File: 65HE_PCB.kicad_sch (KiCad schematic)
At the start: 30 parts, among them J001 JST_SH, SW1 BOOT, SW2 NRST, U201 TLV75733PDBV, U202 TLV75733PDBV, U301 STM32F072CBTx

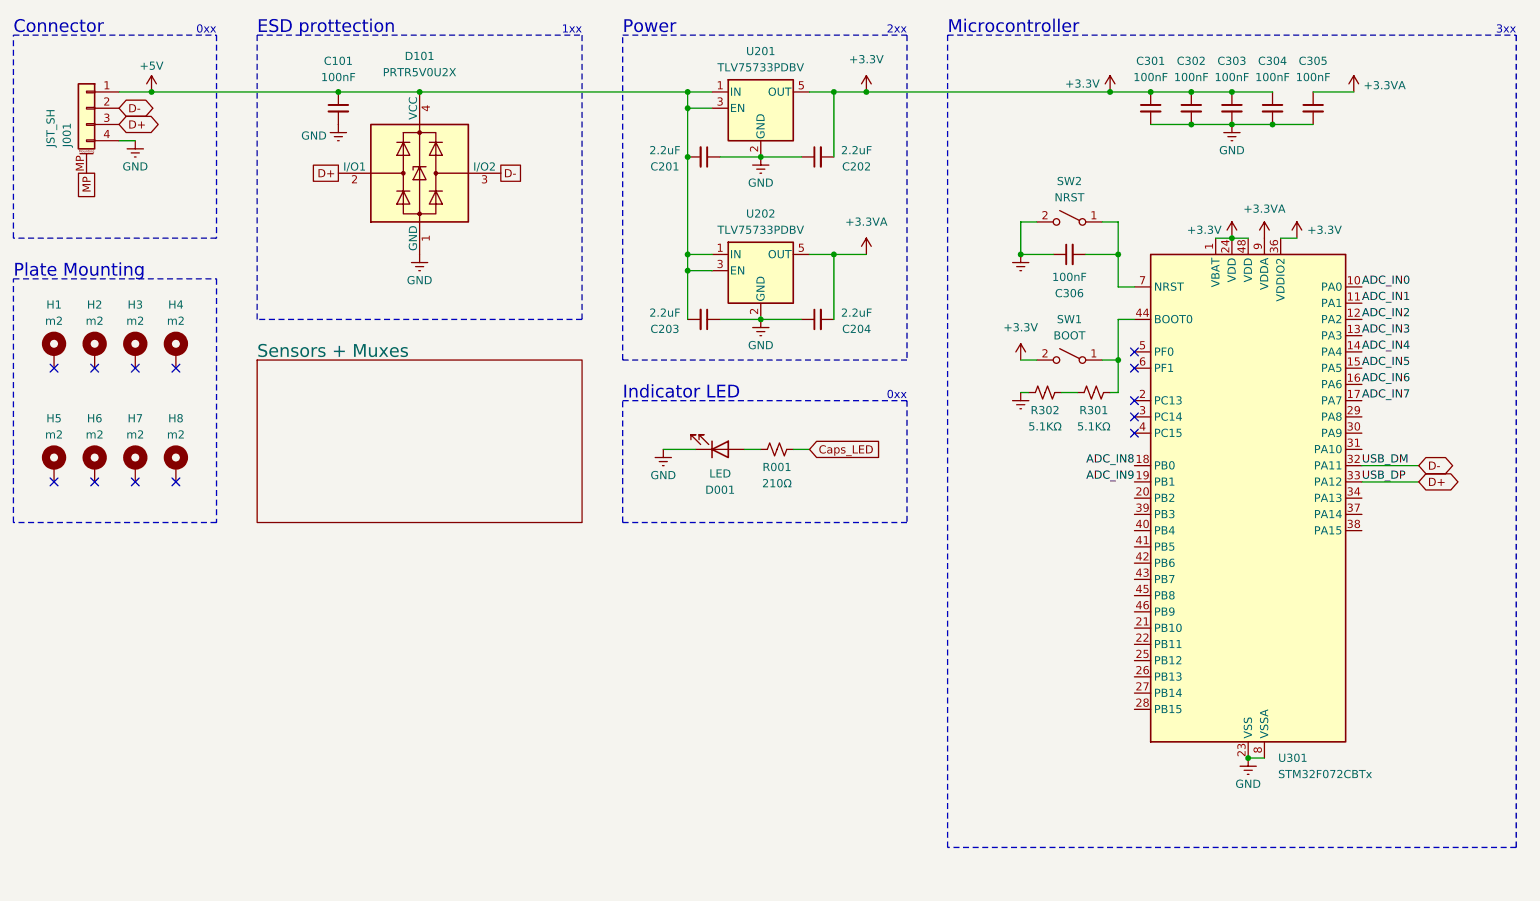
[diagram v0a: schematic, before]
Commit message: initial commit
i made the board yay!
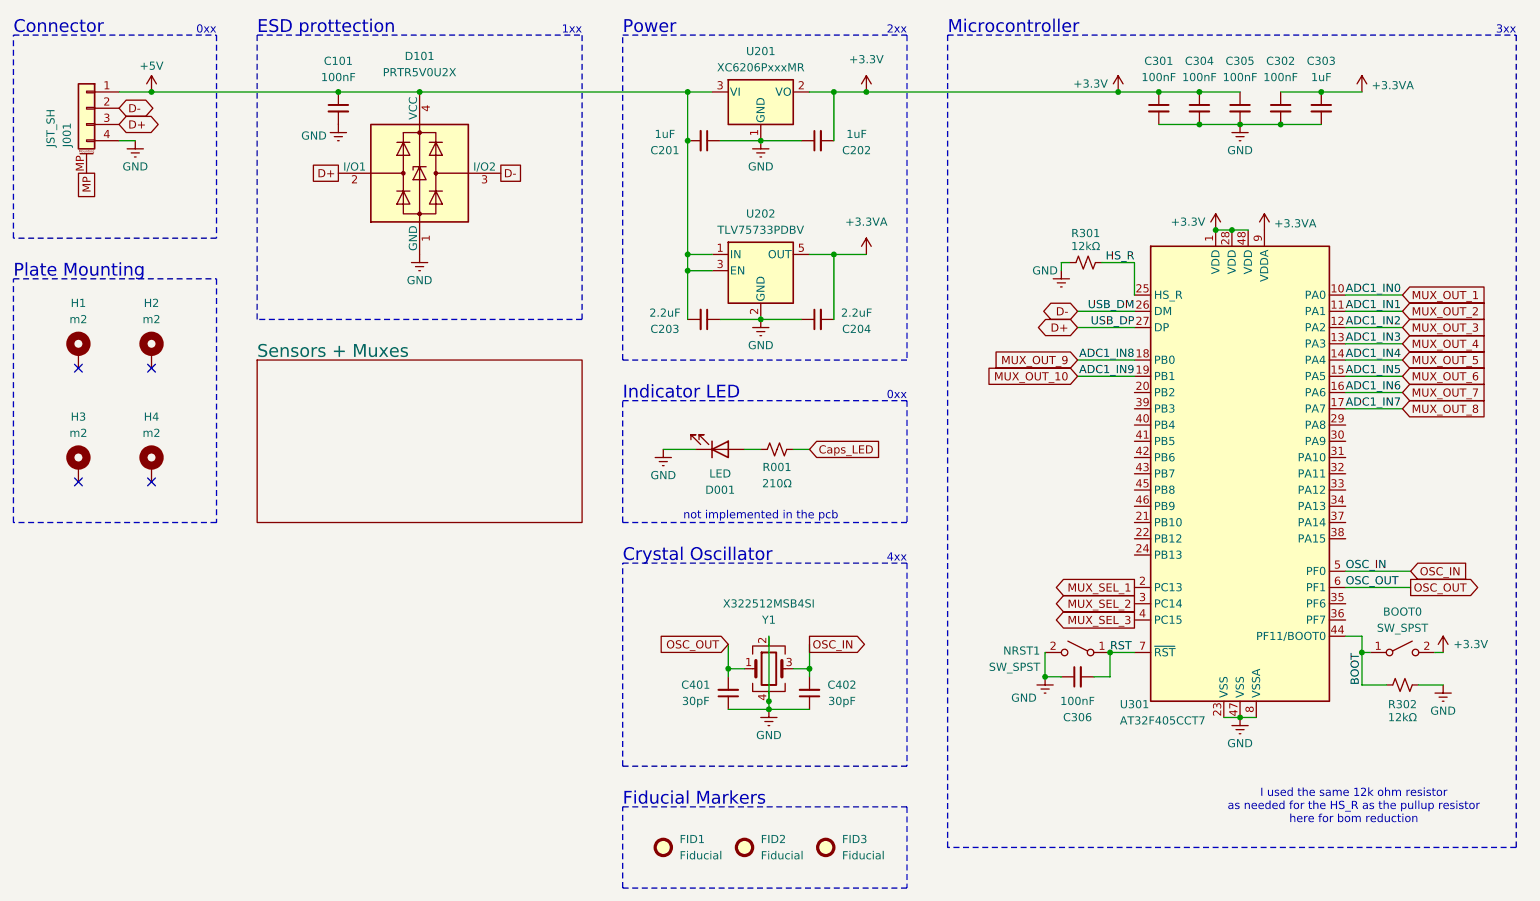
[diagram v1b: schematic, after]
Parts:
- removed C304: 100nF, Capacitor_SMD:C_0805_2012Metric, symbol Device:C_Small
- removed H1, H2, H3, H4, H5, H6, H7, H8: m2, MountingHole:MountingHole_2.2mm_M2_Pad, symbol Mechanical:MountingHole_Pad_MP
- removed SW1: BOOT, PCM_marbastlib-various:SW_SPST_SKQG_WithStem, symbol Switch:SW_SPST
- removed SW2: NRST, PCM_marbastlib-various:SW_SPST_SKQG_WithStem, symbol Switch:SW_SPST
- removed U202: TLV75733PDBV, Package_TO_SOT_SMD:SOT-23-5, symbol Regulator_Linear:TLV75733PDBV
- removed U301: STM32F072CBTx, Package_QFP:LQFP-48_7x7mm_P0.5mm, symbol MCU_ST_STM32F0:STM32F072CBTx
- added BOOT0, NRST1: SW_SPST, PCM_marbastlib-various:SW_SPST_SKQG_WithStem, symbol Switch:SW_SPST
- added C303: 1uF, Capacitor_SMD:C_1206_3216Metric, symbol Device:C_Small
- added C401, C402: 30pF, Capacitor_SMD:C_0603_1608Metric, symbol Device:C_Small
- added FID1, FID2, FID3: Fiducial, Fiducial:Fiducial_1mm_Mask2mm, symbol Mechanical:Fiducial
- added H1, H2, H3, H4: m2, MountingHole:MountingHole_2.2mm_M2_Pad, symbol Mechanical:MountingHole_Pad
- added U201: XC6206PxxxMR, Package_TO_SOT_SMD:SOT-23-3, symbol Regulator_Linear:XC6206PxxxMR
- added U301: AT32F405CCT7, Package_QFP:LQFP-48_7x7mm_P0.5mm, symbol PCM_marbastlib-various:AT32F405CCT7
- added Y1: X322512MSB4SI, Crystal:Crystal_SMD_3225-4Pin_3.2x2.5mm, symbol Device:Crystal_GND24
- C201: renamed from C203; value 2.2uF -> 1uF
- C202: renamed from C204; value 2.2uF -> 1uF
- D001, R001: now left out of the parts list
- R301, R302: value 5.1KΩ -> 12kΩ
- renumbered C201 to C203, C202 to C204, C305 to C302, C302 to C304, C303 to C305, U201 to U202
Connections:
- net +3.3V: now also C202.2, BOOT0.2 (B), U201.2 (VO), U301.1 (VDD), U301.28 (VDD), U301.48 (VDD); no longer C204.2, U202.5 (OUT)
- net +3.3VA: now also C204.2, U202.5 (OUT), C303.1, U301.9 (VDDA); no longer C202.2
- net +5V: now also U201.3 (VI)
- net D+: now also U301.27 (DP)
- net D-: now also U301.26 (DM)
- net GND: now also R301.2, C303.2, C401.1, C402.1, NRST1.2 (B), U201.1 (GND), U301.23 (VSS), U301.47 (VSS), U301.8 (VSSA), Y1.2, Y1.4
- net RST: now reaches C306.2
- net RST: now also NRST1.1 (A), U301.7 (~{RST})
- net BOOT: now reaches R302.2
- net BOOT: now also BOOT0.1 (A), U301.44 (PF11/BOOT0); no longer R301.1
- new net HS_R: R301.1, U301.25 (HS_R)
- new net MUX_OUT_1: U301.10 (PA0)
- new net MUX_OUT_10: U301.19 (PB1)
- new net MUX_OUT_2: U301.11 (PA1)
- new net MUX_OUT_3: U301.12 (PA2)
- new net MUX_OUT_4: U301.13 (PA3)
- new net MUX_OUT_5: U301.14 (PA4)
- new net MUX_OUT_6: U301.15 (PA5)
- new net MUX_OUT_7: U301.16 (PA6)
- new net MUX_OUT_8: U301.17 (PA7)
- new net MUX_OUT_9: U301.18 (PB0)
- new net MUX_SEL_1: U301.2 (PC13)
- new net MUX_SEL_2: U301.3 (PC14)
- new net MUX_SEL_3: U301.4 (PC15)
- new net OSC_IN: C402.2, U301.5 (PF0), Y1.3
- new net OSC_OUT: C401.2, U301.6 (PF1), Y1.1
- no-connect marks 13 -> 4
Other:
- note added: "4xx"
- note added: "Crystal Oscillator"
- note added: "Fiducial Markers"
- note added: "I used the same 12k ohm resistor as needed for the HS_R as the pullup resistor here for bom reduction"
- note added: "not implemented in the pcb"
- moved on the sheet: C201, C202, C203, C204, C301, C302, C304, C305, U202
